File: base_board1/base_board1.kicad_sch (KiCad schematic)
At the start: 99 parts, among them J1 DF40C-60DS-0.4V_51_, J2 DF40C-60DS-0.4V_51_, J3 Conn_01x30, J4 Conn_01x30, J5 Conn_01x30, J6 Conn_01x30

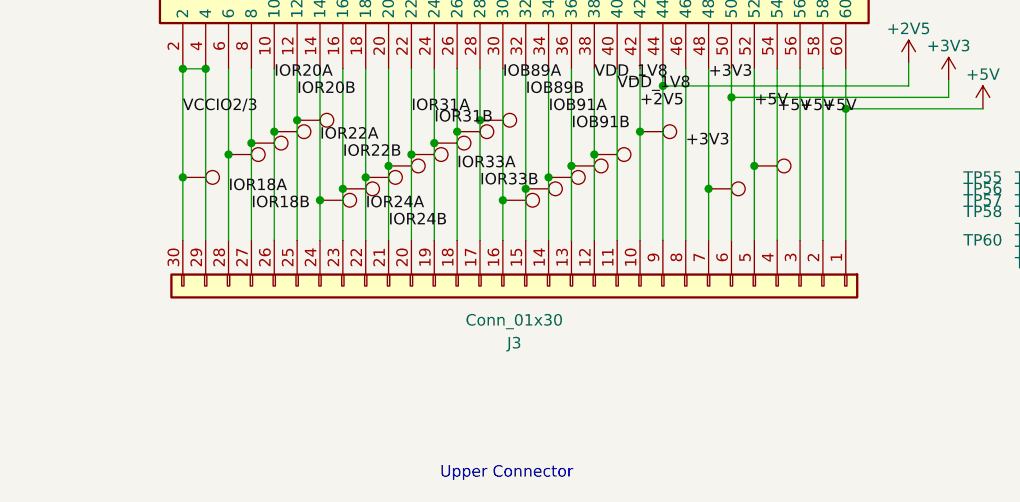
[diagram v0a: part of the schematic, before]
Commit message: 1220
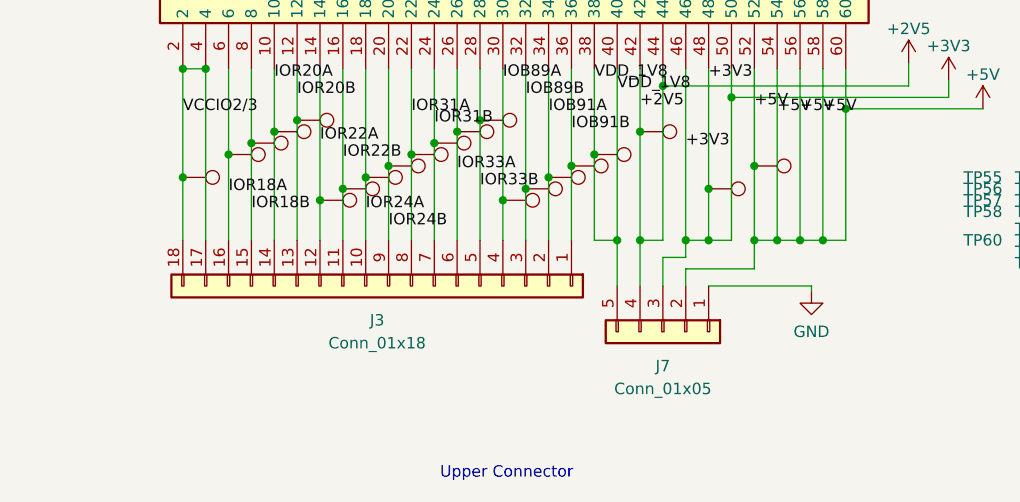
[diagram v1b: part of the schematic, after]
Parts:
- removed J3: Conn_01x30, Connector_PinHeader_2.54mm:PinHeader_1x30_P2.54mm_Vertical_SMD_Pin1Left, symbol Connector_Generic:Conn_01x30
- added J3: Conn_01x18, Connector_PinHeader_2.54mm:PinHeader_1x18_P2.54mm_Vertical_SMD_Pin1Left, symbol Connector_Generic:Conn_01x18
- added J7: Conn_01x05, Connector_PinSocket_2.54mm:PinSocket_1x05_P2.54mm_Vertical, symbol Connector_Generic:Conn_01x05
- TP101, TP103, TP105, TP107, TP109, TP113, TP115, TP117, TP119, TP121, TP123, TP35, TP37, TP40, TP42, TP43, TP44, TP45, TP46, TP47, TP48, TP49, TP50, TP51, TP52, TP53, TP54, TP55, TP56, TP57, TP58, TP60, TP69, TP71, TP73, TP75, TP77, TP79, TP83, TP85, TP87, TP89, TP91, TP95, TP99: footprint TestPoint:TestPoint_Pad_1.5x1.5mm -> TestPoint:TestPoint_THTPad_1.5x1.5mm_Drill0.7mm
- TP11, TP12, TP14, TP15, TP17, TP18, TP19, TP2, TP20, TP22, TP23, TP24, TP25, TP26, TP27, TP28, TP29, TP3, TP30, TP5, TP6, TP8, TP9: footprint TestPoint:TestPoint_THTPad_1.5x1.5mm_Drill0.7mm -> TestPoint:TestPoint_Pad_1.5x1.5mm
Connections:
- net +2V5: now also J7.4 (Pin_4)
- net +3V3: now also J7.3 (Pin_3)
- net +5V: now also J7.2 (Pin_2)
- net GND: now also J7.1 (Pin_1)
- net IOB89A: now also J3.4 (Pin_4)
- net IOB89B: now also J3.3 (Pin_3)
- net IOB91A: now also J3.2 (Pin_2)
- net IOB91B: now also J3.1 (Pin_1)
- net IOR18A: now also J3.16 (Pin_16)
- net IOR18B: now also J3.15 (Pin_15)
- net IOR20A: now also J3.14 (Pin_14)
- net IOR20B: now also J3.13 (Pin_13)
- net IOR22A: now also J3.12 (Pin_12)
- net IOR22B: now also J3.11 (Pin_11)
- net IOR24A: now also J3.10 (Pin_10)
- net IOR24B: now also J3.9 (Pin_9)
- net IOR31A: now also J3.8 (Pin_8)
- net IOR31B: now also J3.7 (Pin_7)
- net IOR33A: now also J3.6 (Pin_6)
- net IOR33B: now also J3.5 (Pin_5)
- net VCCIO2/3: now also J3.17 (Pin_17), J3.18 (Pin_18)
- net VDD_1V8: now also J7.5 (Pin_5)
